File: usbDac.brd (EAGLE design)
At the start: 160 x 100 mm, 3 parts

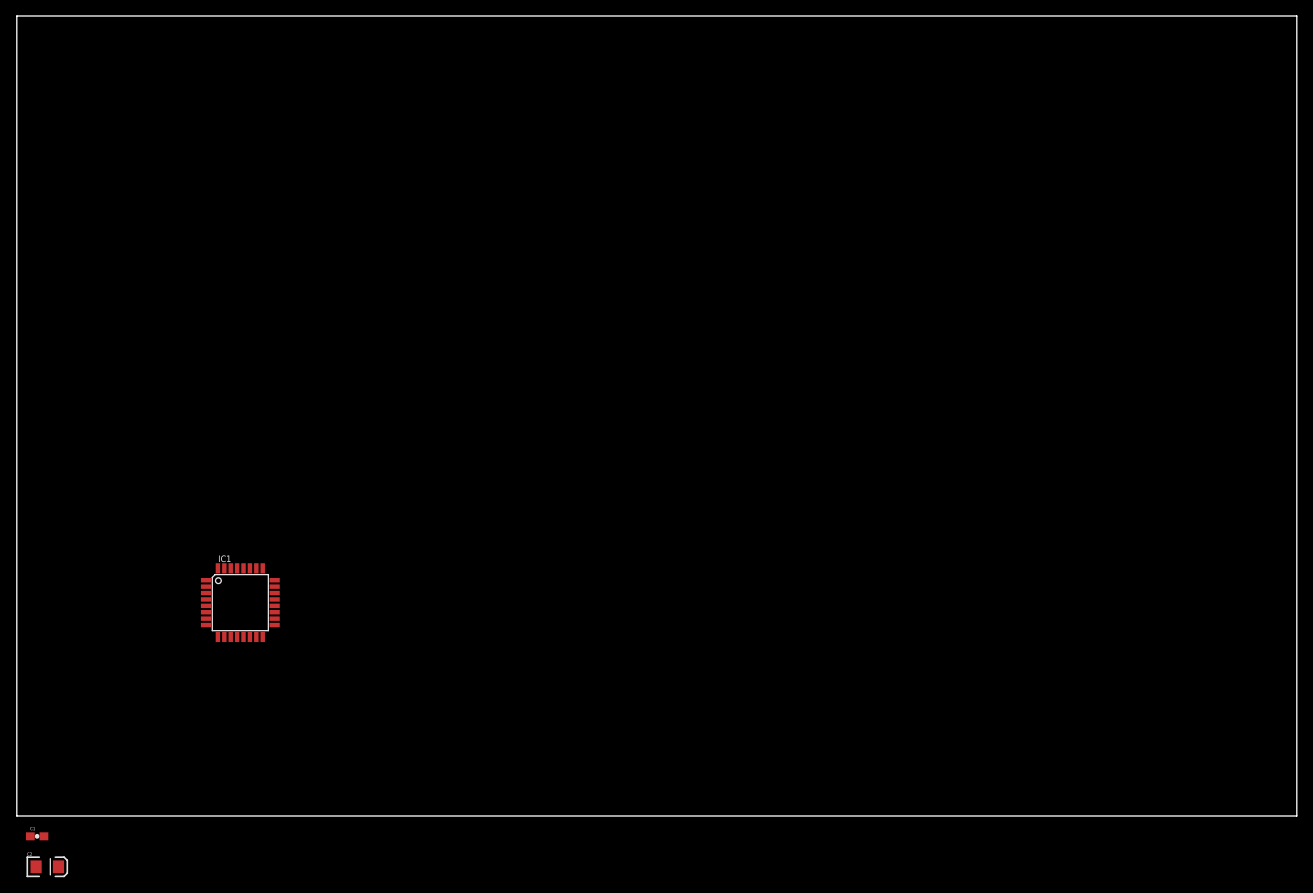
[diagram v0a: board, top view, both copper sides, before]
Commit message: basic routing
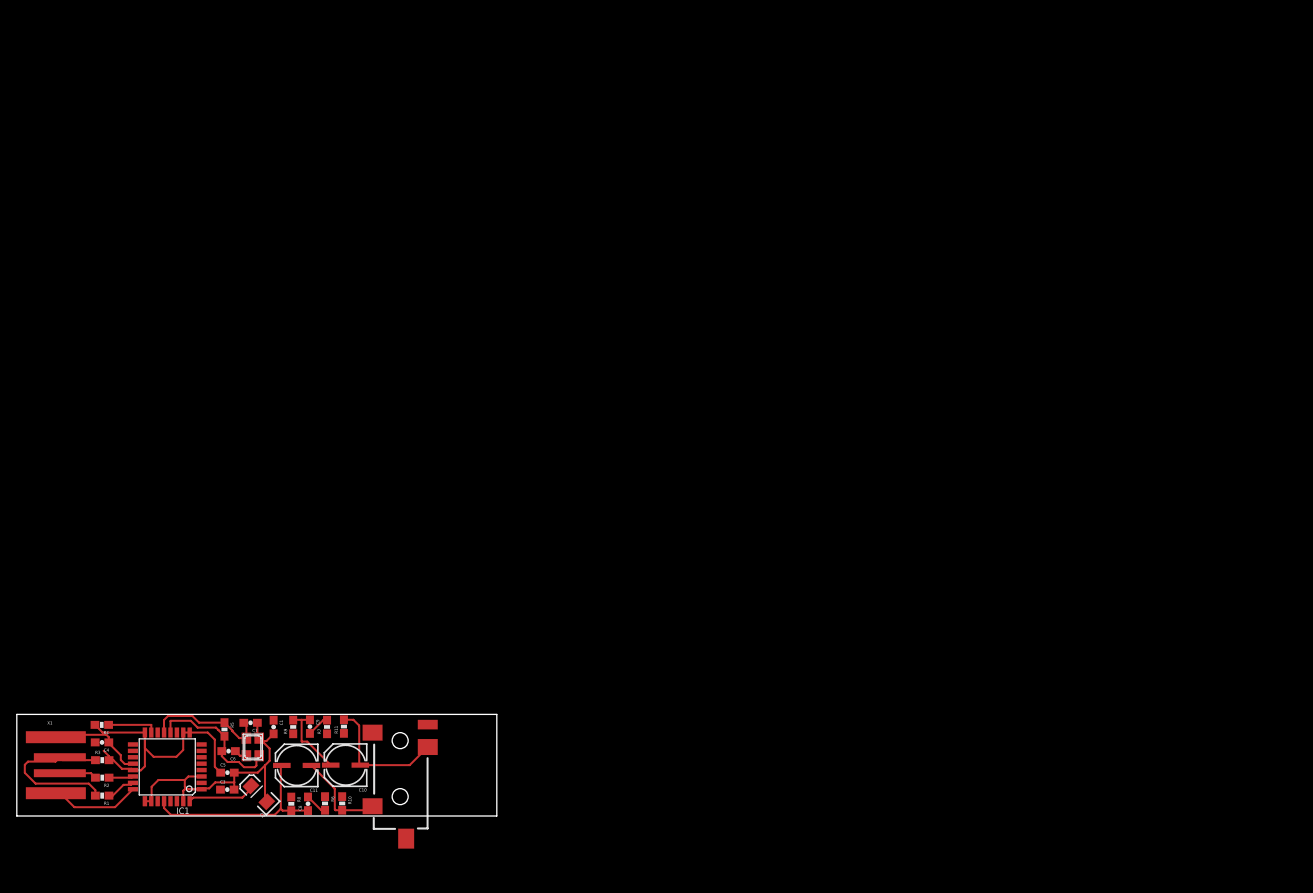
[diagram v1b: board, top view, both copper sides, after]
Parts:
- added C10, C11: 100uF, SparkFun-Capacitors:PANASONIC_C
- added C3, C4, C5, C8, C9: 1uF, SparkFun-Capacitors:0603-CAP
- added C6, C7: (no value), SparkFun-Capacitors:0603-CAP
- added Q1: (no value), adafruit:NX3225
- added R1, R2: 22, SparkFun-Passives:0603-RES
- added R10, R11, R8, R9: 3k3, SparkFun-Passives:0603-RES
- added R3, R4: 1k5, SparkFun-Passives:0603-RES
- added R5: 1M, SparkFun-Passives:0603-RES
- added R6, R7: 16, SparkFun-Passives:0603-RES
- added U1: (no value), SparkFun-Connectors:AUDIO-JACK-3.5MM-SMD
- added X1: USBPCB, SparkFun:USB-A-PCB
- moved C1 32.6 mm to (32.1, 11.1), turned to 270 degrees
- moved C2 28.0 mm to (30.3, 2.77), turned to 135 degrees
- moved IC1 22.5 mm to (18.8, 6.14), turned to 180 degrees
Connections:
- new net MUTE: IC1.6
- new net N$1: C3.1, IC1.30
- new net N$10: C7.2, IC1.13, Q1.3, R5.1
- new net N$11: IC1.15, R4.1
- new net N$12: C10.+, C9.1, IC1.29, R9.2
- new net N$13: C6.1, Q1.4
- new net N$14: C11.+, C8.1, IC1.28, R8.2
- new net N$15: C6.2, IC1.12, Q1.1, R5.2
- new net N$16: C8.2, R6.2
- new net N$17: C9.2, R7.2
- new net N$18: C11.-, R10.2, U1.TIP
- new net N$19: C10.-, R11.2, U1.RING
- new net N$4: C4.2, IC1.27
- new net N$5: IC1.24, X1.5V
- new net N$6: IC1.23, R1.1
- new net N$7: IC1.22, R2.1
- new net N$8: R1.2, R3.1, X1.USB_P
- new net N$9: R2.2, X1.USB_M
- new net PLAY: IC1.5
- new net VDD: C5.1, IC1.10, IC1.16, IC1.21, IC1.9, R3.2, R4.2
- new net VDN: IC1.8
- new net VUP: IC1.7
- net GND: now also C3.2, C4.1, C5.2, C7.1, IC1.31, Q1.2, R10.1, R11.1, R6.1, R7.1, R8.1, R9.1, U1.SLEEVE, X1.GND
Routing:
- net GND: track 0.00 -> 52.0 mm
- net VDD: track 0.00 -> 36.0 mm
- net N$14: track 0.00 -> 25.1 mm
- net N$8: track 0.00 -> 20.8 mm
- net N$15: track 0.00 -> 18.0 mm
- net N$19: track 0.00 -> 16.6 mm
- net N$10: track 0.00 -> 15.3 mm
- net N$18: track 0.00 -> 11.7 mm
- net N$5: track 0.00 -> 11.3 mm
- net N$12: track 0.00 -> 9.66 mm
- net N$3: track 0.00 -> 8.67 mm
- net N$11: track 0.00 -> 6.30 mm
- net N$9: track 0.00 -> 4.68 mm
- net N$6: track 0.00 -> 3.66 mm
- net N$7: track 0.00 -> 3.05 mm
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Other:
- board size 160 x 100 mm -> 60 x 12.7 mm

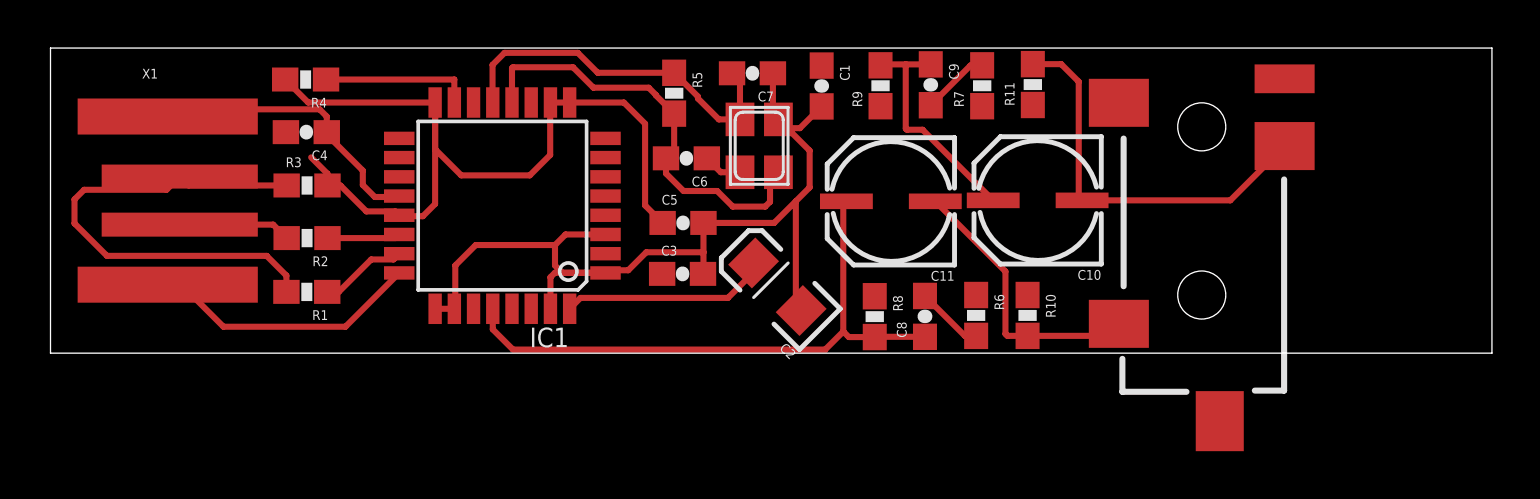
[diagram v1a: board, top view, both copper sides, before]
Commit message: routed
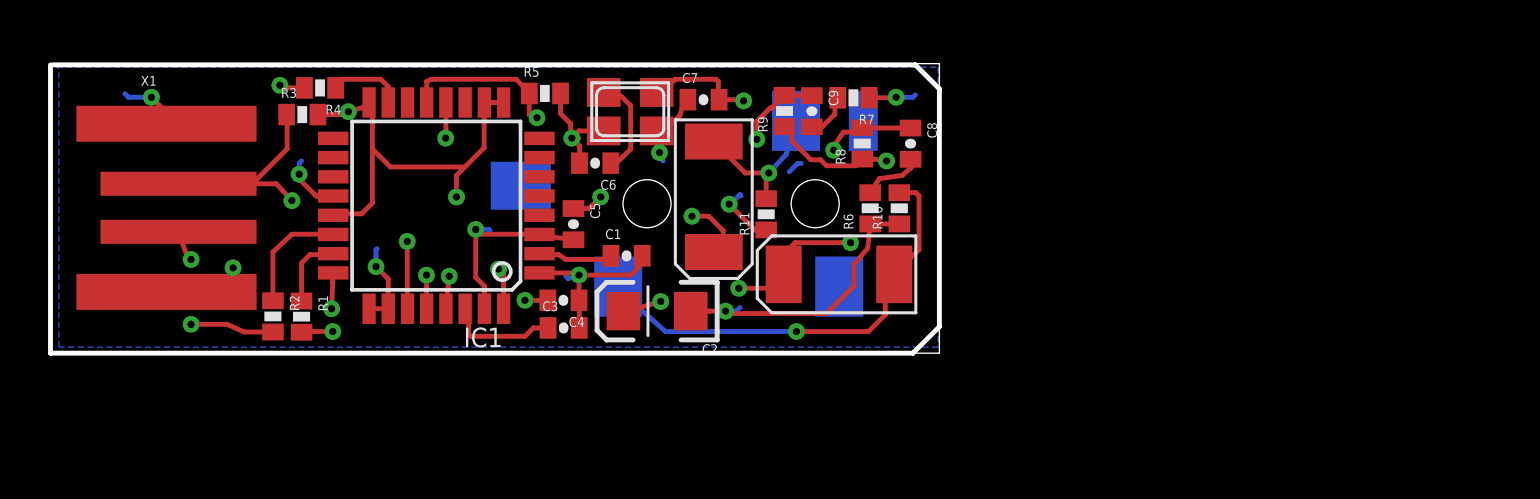
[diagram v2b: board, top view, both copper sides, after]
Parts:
- C1, C3, C4, C5, C6, C7, C8, C9: device SparkFun-Capacitors:0603-CAP -> SparkFun-Capacitors:0402-CAP
- C10, C11: device SparkFun-Capacitors:PANASONIC_C -> SparkFun-Capacitors:EIA6032
- R1, R10, R11, R2, R3, R4, R5, R6, R7, R8, R9: device SparkFun-Passives:0603-RES -> SparkFun-Passives:0402-RES
- moved U1 14.3 mm to (35.3, 6.22), flipped to the bottom, turned to 0 degrees
- moved C10 13.5 mm to (27.6, 6.51), turned to 90 degrees
- moved C4 12.8 mm to (21.4, 2.20)
- moved R11 12.3 mm to (29.8, 5.78)
- moved C1 10.8 mm to (24.0, 4.05), turned to 0 degrees
- moved R8 7.23 mm to (33.8, 8.73), turned to 90 degrees
- moved C8 7.21 mm to (35.8, 8.72), turned to 270 degrees
- moved R10 6.96 mm to (35.3, 6.03), turned to 90 degrees
- moved R6 6.27 mm to (34.1, 6.03), turned to 90 degrees
- moved Q1 5.55 mm to (24.1, 10.1), turned to 0 degrees
- moved C3 5.44 mm to (21.4, 1.05)
- moved R7 5.38 mm to (33.4, 10.6), turned to 180 degrees
- moved R5 5.38 mm to (20.6, 10.8), turned to 0 degrees
- moved C2 5.11 mm to (25.2, 1.75), turned to 180 degrees
- moved C9 5.07 mm to (31.7, 10.1)
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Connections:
- net N$5 renamed VCC
- net N$12: now also C10.P$1; no longer C10.+
- net N$14: now also C11.P$1; no longer C11.+
- net N$18: now also C11.P$2; no longer C11.-
- net N$19: now also C10.P$2; no longer C10.-
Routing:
- net N$12: track 9.66 -> 23.1 mm, vias 0 -> 3
- net N$4: track 0.00 -> 11.2 mm, vias 0 -> 2
- net N$19: track 16.6 -> 7.07 mm, vias 0 -> 1
- net N$18: track 11.7 -> 18.7 mm, vias 0 -> 1
- net VDD: track 36.0 -> 29.5 mm, vias 0 -> 4
- net N$15: track 18.0 -> 11.7 mm, vias 0 -> 2
- net N$10: track 15.3 -> 21.0 mm, vias 0 -> 2
- net N$14: track 25.1 -> 30.7 mm, vias 0 -> 4
- net N$1: track 0.00 -> 4.60 mm
- net N$3: track 8.67 -> 12.2 mm, vias 0 -> 2
- net N$2: track 0.00 -> 3.10 mm
- net N$11: track 6.30 -> 3.23 mm
- net N$9: track 4.68 -> 7.46 mm, vias 0 -> 2
- net N$13: track 1.62 -> 4.22 mm
- net N$7: track 3.05 -> 4.83 mm
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- added copper zone on layer 16, net GND
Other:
- board size 60 x 12.7 mm -> 37 x 12.1 mm
- board text added: "Blinkiverse"
- board text added: "Keep it Locked"
- board text added: "RevA 130314"
- board text added: "blinkiverse.com/microdac"
- board text added: "microDAC"
